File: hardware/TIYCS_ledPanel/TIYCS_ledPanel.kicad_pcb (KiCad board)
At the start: 2 copper layers, 100 x 100 mm, 108 parts

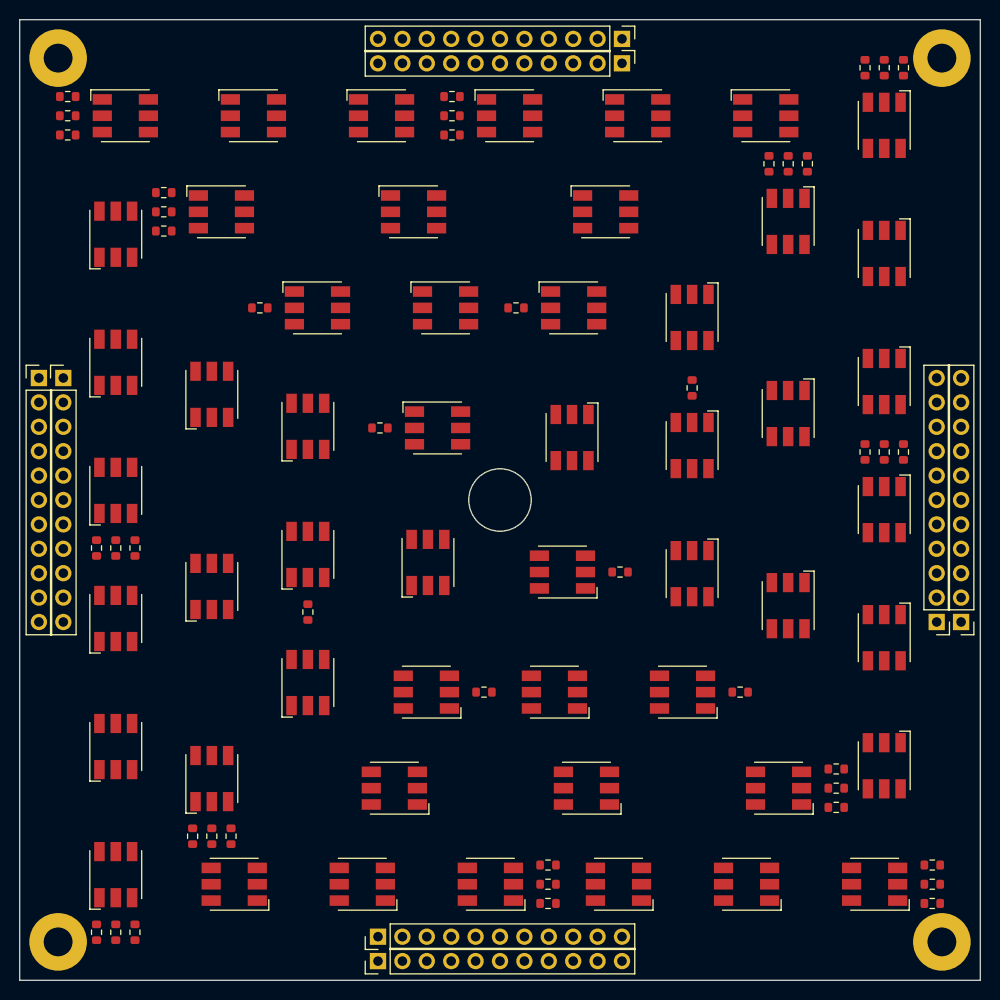
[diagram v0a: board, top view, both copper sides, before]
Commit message: Routed
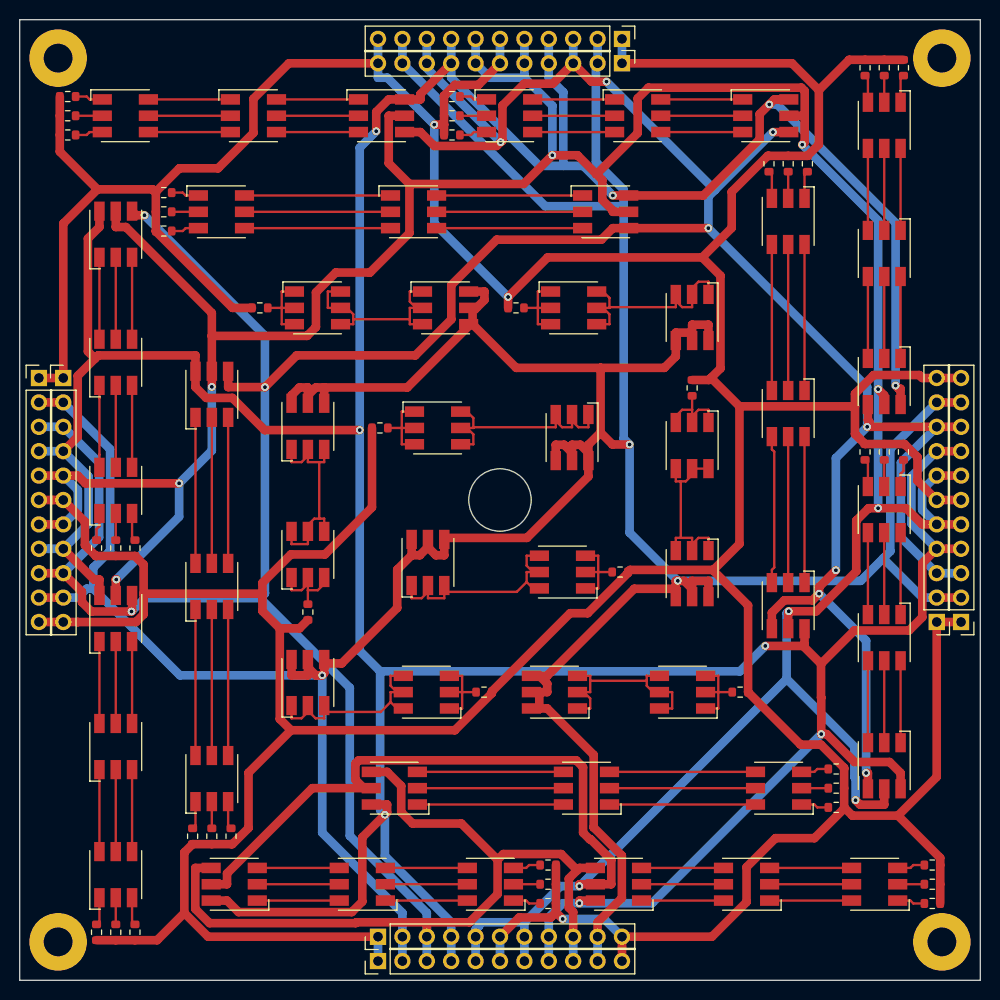
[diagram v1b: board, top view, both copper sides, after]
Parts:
- removed the R_0_0_RGB at (-35.0, -30.0)
- removed the R_0_1_RGB at (-35.0, -32.0)
- removed the R_0_2_RGB at (-35.0, -28.0)
- removed the R_3_0_RGB at (30.0, -35.0)
- removed the R_3_1_RGB at (32.0, -35.0)
- removed the R_3_2_RGB at (28.0, -35.0)
- removed the R_6_0_RGB at (35.0, 30.0)
- removed the R_6_1_RGB at (35.0, 32.0)
- removed the R_6_2_RGB at (35.0, 28.0)
- removed the R_9_0_RGB at (-30.0, 35.0)
- removed the R_9_1_RGB at (-32.0, 35.0)
- removed the R_9_2_RGB at (-28.0, 35.0)
- added R_0_0_RGB2: R_0603_1608Metric, R_0603_1608Metric, F.Cu at (-35.0, -30.0)
- added R_0_1_RGB2: R_0603_1608Metric, R_0603_1608Metric, F.Cu at (-35.0, -32.0)
- added R_0_2_RGB2: R_0603_1608Metric, R_0603_1608Metric, F.Cu at (-35.0, -28.0)
- added R_3_0_RGB2: R_0603_1608Metric, R_0603_1608Metric, F.Cu at (30.0, -35.0)
- added R_3_1_RGB2: R_0603_1608Metric, R_0603_1608Metric, F.Cu at (32.0, -35.0)
- added R_3_2_RGB2: R_0603_1608Metric, R_0603_1608Metric, F.Cu at (28.0, -35.0)
- added R_6_0_RGB2: R_0603_1608Metric, R_0603_1608Metric, F.Cu at (35.0, 30.0)
- added R_6_1_RGB2: R_0603_1608Metric, R_0603_1608Metric, F.Cu at (35.0, 32.0)
- added R_6_2_RGB2: R_0603_1608Metric, R_0603_1608Metric, F.Cu at (35.0, 28.0)
- added R_9_0_RGB2: R_0603_1608Metric, R_0603_1608Metric, F.Cu at (-30.0, 35.0)
- added R_9_1_RGB2: R_0603_1608Metric, R_0603_1608Metric, F.Cu at (-32.0, 35.0)
- added R_9_2_RGB2: R_0603_1608Metric, R_0603_1608Metric, F.Cu at (-28.0, 35.0)
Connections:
- net D10toD11_W renamed D10toD11_W_1
- net D12toD13_Blue renamed D12toD13_Blue_1
- net D12toD13_Green renamed D12toD13_Green_1
- net D12toD13_Red renamed D12toD13_Red_1
- net D13toD14_Blue renamed D13toD14_Blue_1
- net D13toD14_Green renamed D13toD14_Green_1
- net D13toD14_Red renamed D13toD14_Red_1
- net D15toD16_Blue renamed D15toD16_Blue_1
- net D15toD16_Green renamed D15toD16_Green_1
- net D15toD16_Red renamed D15toD16_Red_1
- net D16toD17_Blue renamed D16toD17_Blue_1
- net D16toD17_Green renamed D16toD17_Green_1
- net D16toD17_Red renamed D16toD17_Red_1
- net D18toD19_Blue renamed D18toD19_Blue_1
- net D18toD19_Green renamed D18toD19_Green_1
- net D18toD19_Red renamed D18toD19_Red_1
- net D19toD20_Blue renamed D19toD20_Blue_1
- net D19toD20_Green renamed D19toD20_Green_1
- net D19toD20_Red renamed D19toD20_Red_1
- net D21toD22_Blue renamed D21toD22_Blue_1
- net D21toD22_Green renamed D21toD22_Green_1
- net D21toD22_Red renamed D21toD22_Red_1
- net D22toD23_Blue renamed D22toD23_Blue_1
- net D22toD23_Green renamed D22toD23_Green_1
- net D22toD23_Red renamed D22toD23_Red_1
- net D4toD5_W renamed D4toD5_W_1
- net D6toD7_W renamed D6toD7_W_1
- net D8toD9_W renamed D8toD9_W_1
- net RtoD10_W renamed RtoD10_W_1
- net RtoD12_Blue renamed RtoD12_Blue_1
- net RtoD12_Green renamed RtoD12_Green_1
- net RtoD12_Red renamed RtoD12_Red_1
- net RtoD15_Blue renamed RtoD15_Blue_1
- net RtoD15_Green renamed RtoD15_Green_1
- net RtoD15_Red renamed RtoD15_Red_1
- net RtoD18_Blue renamed RtoD18_Blue_1
- net RtoD18_Green renamed RtoD18_Green_1
- net RtoD18_Red renamed RtoD18_Red_1
- net RtoD21_Blue renamed RtoD21_Blue_1
- net RtoD21_Green renamed RtoD21_Green_1
- net RtoD21_Red renamed RtoD21_Red_1
- net RtoD4_W renamed RtoD4_W_1
- net RtoD6_W renamed RtoD6_W_1
- net RtoD8_W renamed RtoD8_W_1
- LED_RGB2_0 pad 1: RtoD0_Green -> RtoD0_Green_2
- LED_RGB2_0 pad 2: RtoD0_Red -> RtoD0_Red_2
- LED_RGB2_0 pad 3: RtoD0_Blue -> RtoD0_Blue_2
- LED_RGB2_0 pad 4: D0toD1_Blue -> D0toD1_Blue_2
- LED_RGB2_0 pad 5: D0toD1_Red -> D0toD1_Red_2
- LED_RGB2_0 pad 6: D0toD1_Green -> D0toD1_Green_2
- LED_RGB2_1 pad 1: D0toD1_Green -> D0toD1_Green_2
- LED_RGB2_1 pad 2: D0toD1_Red -> D0toD1_Red_2
- LED_RGB2_1 pad 3: D0toD1_Blue -> D0toD1_Blue_2
- LED_RGB2_1 pad 4: D1toD2_Blue -> D1toD2_Blue_2
- LED_RGB2_1 pad 5: D1toD2_Red -> D1toD2_Red_2
- LED_RGB2_1 pad 6: D1toD2_Green -> D1toD2_Green_2
- LED_RGB2_10 pad 1: D9toD10_Green -> D9toD10_Green_2
- LED_RGB2_10 pad 2: D9toD10_Red -> D9toD10_Red_2
- LED_RGB2_10 pad 3: D9toD10_Blue -> D9toD10_Blue_2
- LED_RGB2_10 pad 4: D10toD11_Blue -> D10toD11_Blue_2
- LED_RGB2_10 pad 5: D10toD11_Red -> D10toD11_Red_2
- LED_RGB2_10 pad 6: D10toD11_Green -> D10toD11_Green_2
- LED_RGB2_11 pad 1: D10toD11_Green -> D10toD11_Green_2
- LED_RGB2_11 pad 2: D10toD11_Red -> D10toD11_Red_2
- LED_RGB2_11 pad 3: D10toD11_Blue -> D10toD11_Blue_2
- LED_RGB2_2 pad 1: D1toD2_Green -> D1toD2_Green_2
- LED_RGB2_2 pad 2: D1toD2_Red -> D1toD2_Red_2
- LED_RGB2_2 pad 3: D1toD2_Blue -> D1toD2_Blue_2
- LED_RGB2_3 pad 1: RtoD3_Green -> RtoD3_Green_2
- LED_RGB2_3 pad 2: RtoD3_Red -> RtoD3_Red_2
- LED_RGB2_3 pad 3: RtoD3_Blue -> RtoD3_Blue_2
- LED_RGB2_3 pad 4: D3toD4_Blue -> D3toD4_Blue_2
- LED_RGB2_3 pad 5: D3toD4_Red -> D3toD4_Red_2
- LED_RGB2_3 pad 6: D3toD4_Green -> D3toD4_Green_2
- LED_RGB2_4 pad 1: D3toD4_Green -> D3toD4_Green_2
- LED_RGB2_4 pad 2: D3toD4_Red -> D3toD4_Red_2
- LED_RGB2_4 pad 3: D3toD4_Blue -> D3toD4_Blue_2
- LED_RGB2_4 pad 4: D4toD5_Blue -> D4toD5_Blue_2
- LED_RGB2_4 pad 5: D4toD5_Red -> D4toD5_Red_2
- LED_RGB2_4 pad 6: D4toD5_Green -> D4toD5_Green_2
- LED_RGB2_5 pad 1: D4toD5_Green -> D4toD5_Green_2
- LED_RGB2_5 pad 2: D4toD5_Red -> D4toD5_Red_2
- LED_RGB2_5 pad 3: D4toD5_Blue -> D4toD5_Blue_2
- LED_RGB2_6 pad 1: RtoD6_Green -> RtoD6_Green_2
- LED_RGB2_6 pad 2: RtoD6_Red -> RtoD6_Red_2
- LED_RGB2_6 pad 3: RtoD6_Blue -> RtoD6_Blue_2
- LED_RGB2_6 pad 4: D6toD7_Blue -> D6toD7_Blue_2
- LED_RGB2_6 pad 5: D6toD7_Red -> D6toD7_Red_2
- LED_RGB2_6 pad 6: D6toD7_Green -> D6toD7_Green_2
- LED_RGB2_7 pad 1: D6toD7_Green -> D6toD7_Green_2
- LED_RGB2_7 pad 2: D6toD7_Red -> D6toD7_Red_2
- LED_RGB2_7 pad 3: D6toD7_Blue -> D6toD7_Blue_2
- LED_RGB2_7 pad 4: D7toD8_Blue -> D7toD8_Blue_2
- LED_RGB2_7 pad 5: D7toD8_Red -> D7toD8_Red_2
- LED_RGB2_7 pad 6: D7toD8_Green -> D7toD8_Green_2
- LED_RGB2_8 pad 1: D7toD8_Green -> D7toD8_Green_2
- LED_RGB2_8 pad 2: D7toD8_Red -> D7toD8_Red_2
- LED_RGB2_8 pad 3: D7toD8_Blue -> D7toD8_Blue_2
- LED_RGB2_9 pad 1: RtoD9_Green -> RtoD9_Green_2
- LED_RGB2_9 pad 2: RtoD9_Red -> RtoD9_Red_2
- LED_RGB2_9 pad 3: RtoD9_Blue -> RtoD9_Blue_2
- LED_RGB2_9 pad 4: D9toD10_Blue -> D9toD10_Blue_2
- LED_RGB2_9 pad 5: D9toD10_Red -> D9toD10_Red_2
- LED_RGB2_9 pad 6: D9toD10_Green -> D9toD10_Green_2
- LED_RGB_0 pad 1: RtoD0_Green -> RtoD0_Green_1
- LED_RGB_0 pad 2: RtoD0_Red -> RtoD0_Red_1
- LED_RGB_0 pad 3: RtoD0_Blue -> RtoD0_Blue_1
- LED_RGB_0 pad 4: D0toD1_Blue -> D0toD1_Blue_1
- LED_RGB_0 pad 5: D0toD1_Red -> D0toD1_Red_1
- LED_RGB_0 pad 6: D0toD1_Green -> D0toD1_Green_1
- LED_RGB_1 pad 1: D0toD1_Green -> D0toD1_Green_1
- LED_RGB_1 pad 2: D0toD1_Red -> D0toD1_Red_1
- LED_RGB_1 pad 3: D0toD1_Blue -> D0toD1_Blue_1
- LED_RGB_1 pad 4: D1toD2_Blue -> D1toD2_Blue_1
- LED_RGB_1 pad 5: D1toD2_Red -> D1toD2_Red_1
- LED_RGB_1 pad 6: D1toD2_Green -> D1toD2_Green_1
- LED_RGB_10 pad 1: D9toD10_Green -> D9toD10_Green_1
- LED_RGB_10 pad 2: D9toD10_Red -> D9toD10_Red_1
- LED_RGB_10 pad 3: D9toD10_Blue -> D9toD10_Blue_1
- LED_RGB_10 pad 4: D10toD11_Blue -> D10toD11_Blue_1
- LED_RGB_10 pad 5: D10toD11_Red -> D10toD11_Red_1
- LED_RGB_10 pad 6: D10toD11_Green -> D10toD11_Green_1
- LED_RGB_11 pad 1: D10toD11_Green -> D10toD11_Green_1
- LED_RGB_11 pad 2: D10toD11_Red -> D10toD11_Red_1
- LED_RGB_11 pad 3: D10toD11_Blue -> D10toD11_Blue_1
- LED_RGB_2 pad 1: D1toD2_Green -> D1toD2_Green_1
- LED_RGB_2 pad 2: D1toD2_Red -> D1toD2_Red_1
- LED_RGB_2 pad 3: D1toD2_Blue -> D1toD2_Blue_1
- LED_RGB_3 pad 1: RtoD3_Green -> RtoD3_Green_1
- LED_RGB_3 pad 2: RtoD3_Red -> RtoD3_Red_1
- LED_RGB_3 pad 3: RtoD3_Blue -> RtoD3_Blue_1
- LED_RGB_3 pad 4: D3toD4_Blue -> D3toD4_Blue_1
- LED_RGB_3 pad 5: D3toD4_Red -> D3toD4_Red_1
- LED_RGB_3 pad 6: D3toD4_Green -> D3toD4_Green_1
- LED_RGB_4 pad 1: D3toD4_Green -> D3toD4_Green_1
- LED_RGB_4 pad 2: D3toD4_Red -> D3toD4_Red_1
- LED_RGB_4 pad 3: D3toD4_Blue -> D3toD4_Blue_1
- LED_RGB_4 pad 4: D4toD5_Blue -> D4toD5_Blue_1
- LED_RGB_4 pad 5: D4toD5_Red -> D4toD5_Red_1
- LED_RGB_4 pad 6: D4toD5_Green -> D4toD5_Green_1
- LED_RGB_5 pad 1: D4toD5_Green -> D4toD5_Green_1
- LED_RGB_5 pad 2: D4toD5_Red -> D4toD5_Red_1
- LED_RGB_5 pad 3: D4toD5_Blue -> D4toD5_Blue_1
- LED_RGB_6 pad 1: RtoD6_Green -> RtoD6_Green_1
- LED_RGB_6 pad 2: RtoD6_Red -> RtoD6_Red_1
- LED_RGB_6 pad 3: RtoD6_Blue -> RtoD6_Blue_1
- LED_RGB_6 pad 4: D6toD7_Blue -> D6toD7_Blue_1
- LED_RGB_6 pad 5: D6toD7_Red -> D6toD7_Red_1
- LED_RGB_6 pad 6: D6toD7_Green -> D6toD7_Green_1
- LED_RGB_7 pad 1: D6toD7_Green -> D6toD7_Green_1
- LED_RGB_7 pad 2: D6toD7_Red -> D6toD7_Red_1
- LED_RGB_7 pad 3: D6toD7_Blue -> D6toD7_Blue_1
- LED_RGB_7 pad 4: D7toD8_Blue -> D7toD8_Blue_1
- LED_RGB_7 pad 5: D7toD8_Red -> D7toD8_Red_1
- LED_RGB_7 pad 6: D7toD8_Green -> D7toD8_Green_1
- LED_RGB_8 pad 1: D7toD8_Green -> D7toD8_Green_1
- LED_RGB_8 pad 2: D7toD8_Red -> D7toD8_Red_1
- LED_RGB_8 pad 3: D7toD8_Blue -> D7toD8_Blue_1
- LED_RGB_9 pad 1: RtoD9_Green -> RtoD9_Green_1
- LED_RGB_9 pad 2: RtoD9_Red -> RtoD9_Red_1
- LED_RGB_9 pad 3: RtoD9_Blue -> RtoD9_Blue_1
- LED_RGB_9 pad 4: D9toD10_Blue -> D9toD10_Blue_1
- LED_RGB_9 pad 5: D9toD10_Red -> D9toD10_Red_1
- LED_RGB_9 pad 6: D9toD10_Green -> D9toD10_Green_1
- LED_W2_0 pad 1: RtoD0_W -> RtoD0_W_2
- LED_W2_0 pad 2: RtoD0_W -> RtoD0_W_2
- LED_W2_0 pad 3: RtoD0_W -> RtoD0_W_2
- LED_W2_0 pad 4: D0toD1_W -> D0toD1_W_2
- LED_W2_0 pad 5: D0toD1_W -> D0toD1_W_2
- LED_W2_0 pad 6: D0toD1_W -> D0toD1_W_2
- LED_W2_1 pad 1: D0toD1_W -> D0toD1_W_2
- LED_W2_1 pad 2: D0toD1_W -> D0toD1_W_2
- LED_W2_1 pad 3: D0toD1_W -> D0toD1_W_2
- LED_W2_2 pad 1: RtoD2_W -> RtoD2_W_2
- LED_W2_2 pad 2: RtoD2_W -> RtoD2_W_2
- LED_W2_2 pad 3: RtoD2_W -> RtoD2_W_2
- LED_W2_2 pad 4: D2toD3_W -> D2toD3_W_2
- LED_W2_2 pad 5: D2toD3_W -> D2toD3_W_2
- LED_W2_2 pad 6: D2toD3_W -> D2toD3_W_2
- LED_W2_3 pad 1: D2toD3_W -> D2toD3_W_2
- LED_W2_3 pad 2: D2toD3_W -> D2toD3_W_2
- LED_W2_3 pad 3: D2toD3_W -> D2toD3_W_2
- LED_W_0 pad 1: RtoD0_W -> RtoD0_W_1
- LED_W_0 pad 2: RtoD0_W -> RtoD0_W_1
- LED_W_0 pad 3: RtoD0_W -> RtoD0_W_1
- LED_W_0 pad 4: D0toD1_W -> D0toD1_W_1
- LED_W_0 pad 5: D0toD1_W -> D0toD1_W_1
- LED_W_0 pad 6: D0toD1_W -> D0toD1_W_1
- LED_W_1 pad 1: D0toD1_W -> D0toD1_W_1
- LED_W_1 pad 2: D0toD1_W -> D0toD1_W_1
- LED_W_1 pad 3: D0toD1_W -> D0toD1_W_1
- LED_W_2 pad 1: RtoD2_W -> RtoD2_W_1
- LED_W_2 pad 2: RtoD2_W -> RtoD2_W_1
- LED_W_2 pad 3: RtoD2_W -> RtoD2_W_1
- LED_W_2 pad 4: D2toD3_W -> D2toD3_W_1
- LED_W_2 pad 5: D2toD3_W -> D2toD3_W_1
- LED_W_2 pad 6: D2toD3_W -> D2toD3_W_1
- LED_W_3 pad 1: D2toD3_W -> D2toD3_W_1
- LED_W_3 pad 2: D2toD3_W -> D2toD3_W_1
- LED_W_3 pad 3: D2toD3_W -> D2toD3_W_1
- R_0_0_RGB pad 2: RtoD0_Red -> RtoD0_Red_1
- R_0_0_W pad 2: RtoD0_W -> RtoD0_W_1
- R_0_0_W2 pad 2: RtoD0_W -> RtoD0_W_2
- R_0_1_RGB pad 2: RtoD0_Green -> RtoD0_Green_1
- R_0_2_RGB pad 2: RtoD0_Blue -> RtoD0_Blue_1
- R_2_0_W pad 2: RtoD2_W -> RtoD2_W_1
- R_2_0_W2 pad 2: RtoD2_W -> RtoD2_W_2
- R_3_0_RGB pad 2: RtoD3_Red -> RtoD3_Red_1
- R_3_1_RGB pad 2: RtoD3_Green -> RtoD3_Green_1
- R_3_2_RGB pad 2: RtoD3_Blue -> RtoD3_Blue_1
- R_6_0_RGB pad 2: RtoD6_Red -> RtoD6_Red_1
- R_6_1_RGB pad 2: RtoD6_Green -> RtoD6_Green_1
- R_6_2_RGB pad 2: RtoD6_Blue -> RtoD6_Blue_1
- R_9_0_RGB pad 2: RtoD9_Red -> RtoD9_Red_1
- R_9_1_RGB pad 2: RtoD9_Green -> RtoD9_Green_1
- R_9_2_RGB pad 2: RtoD9_Blue -> RtoD9_Blue_1
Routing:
- net 12V: track 0.00 -> 627.5 mm, vias 0 -> 3
- net B: track 0.00 -> 469.9 mm, vias 0 -> 11
- net G: track 0.00 -> 467.2 mm, vias 0 -> 9
- net W: track 0.00 -> 440.6 mm, vias 0 -> 3
- net R: track 0.00 -> 422.9 mm, vias 0 -> 10
- net D2toD3_W_2: track 0.00 -> 23.9 mm
- net D0toD1_W_2: track 0.00 -> 23.8 mm
- net D2toD3_W_1: track 0.00 -> 22.8 mm
- net D8toD9_W_1: track 0.00 -> 21.9 mm
- net D10toD11_W_1: track 0.00 -> 21.8 mm
- net D0toD1_W_1: track 0.00 -> 21.8 mm
- net D6toD7_W_1: track 0.00 -> 21.8 mm
- net D4toD5_W_1: track 0.00 -> 19.2 mm
- net D4toD5_Blue_2: track 0.00 -> 15.4 mm
- net D9toD10_Red_2: track 0.00 -> 15.2 mm
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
